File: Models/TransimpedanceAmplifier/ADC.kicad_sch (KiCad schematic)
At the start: 9 parts, among them U13 ADS8699

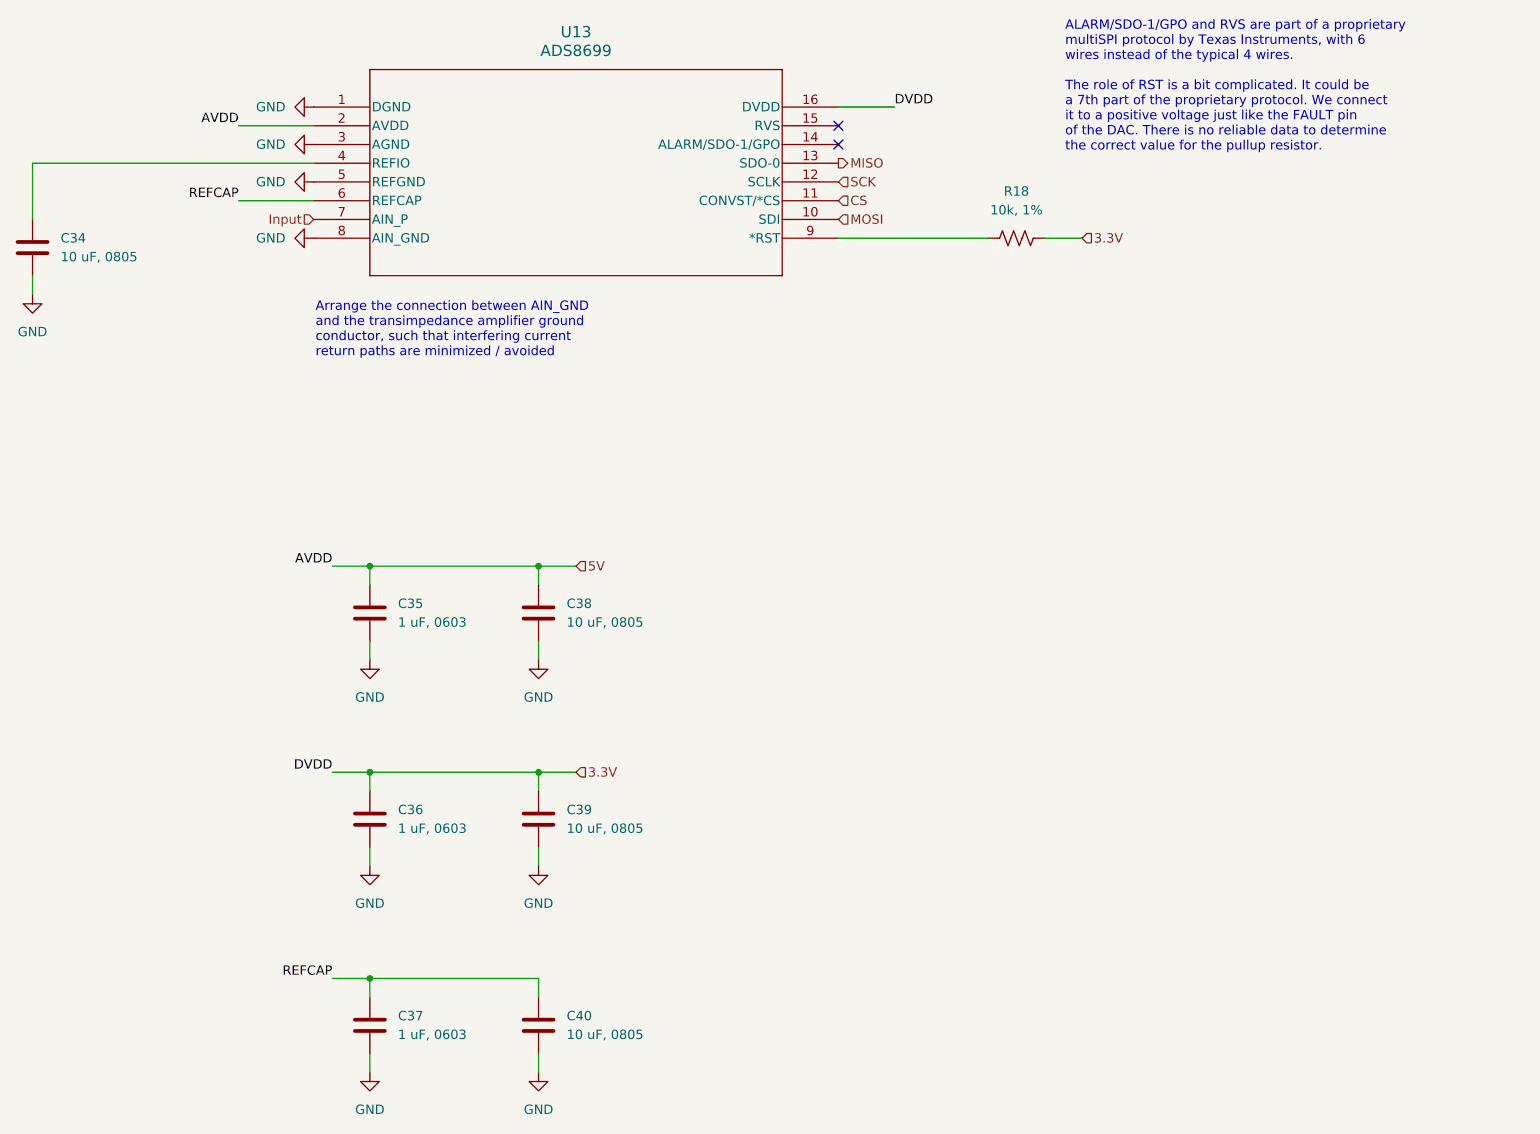
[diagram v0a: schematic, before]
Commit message: First successful ERC
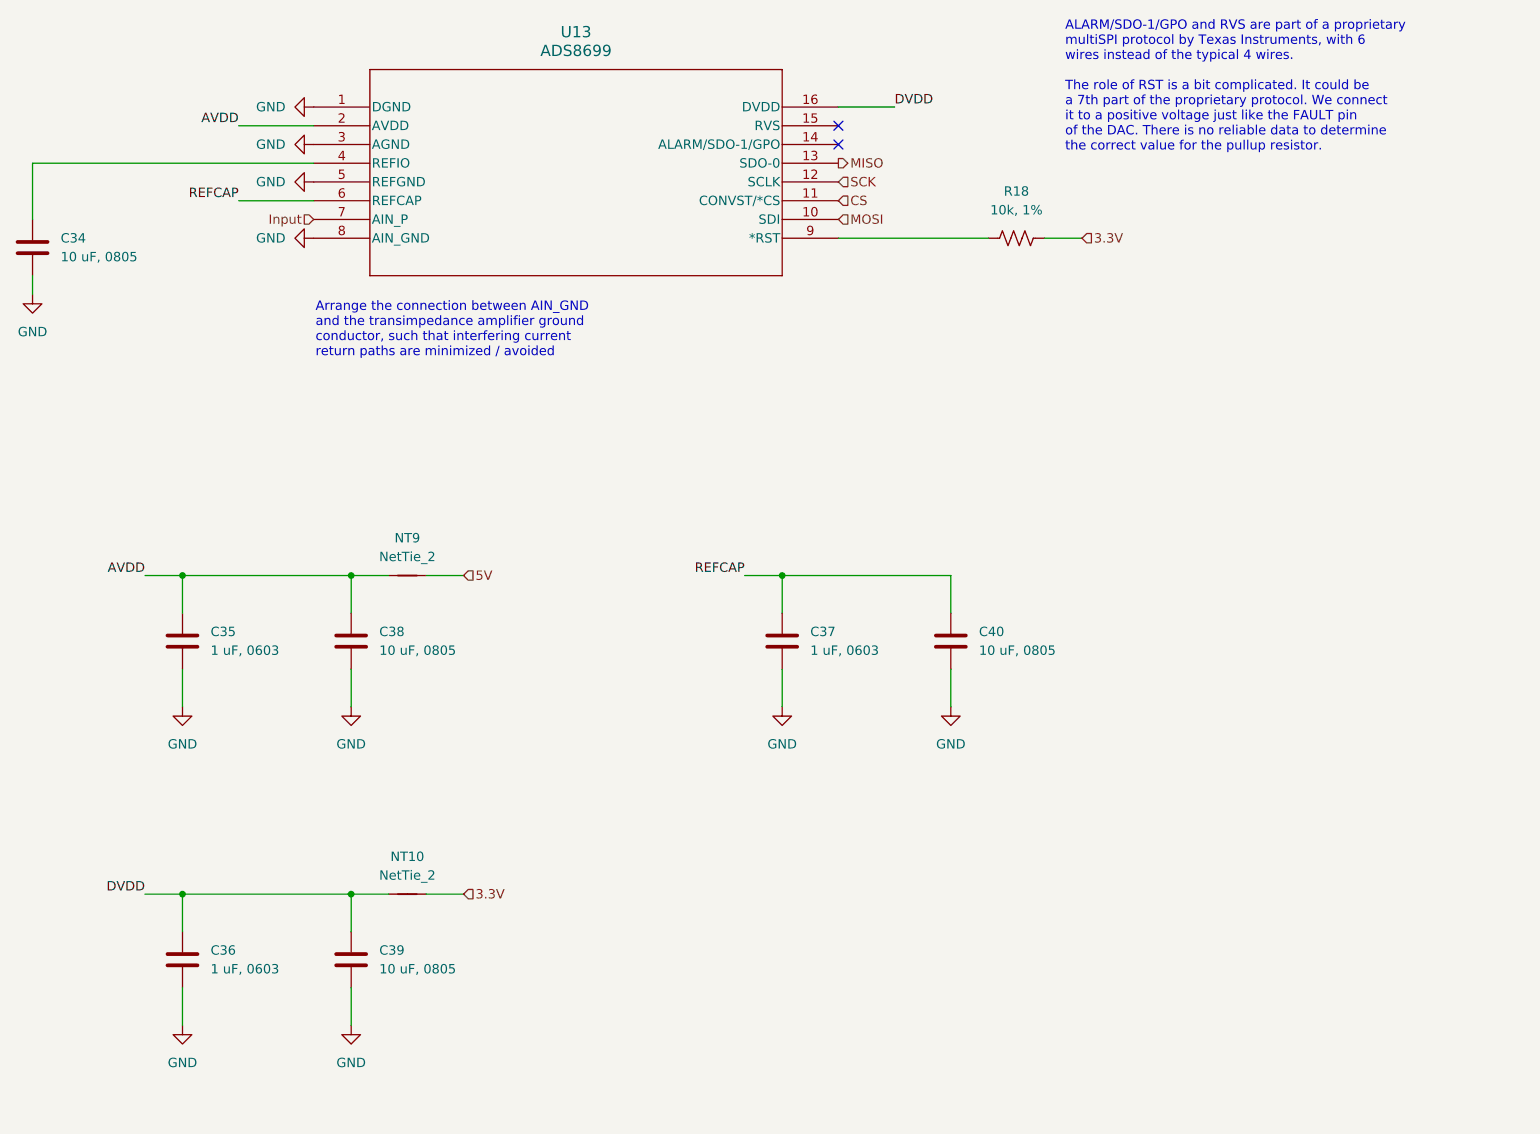
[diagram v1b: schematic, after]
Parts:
- added NT10, NT9: NetTie_2, symbol Device:NetTie_2
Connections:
- net 3.3V: now also NT10.2; no longer C36.1, C39.1, U13.16 (DVDD)
- net 5V: now also NT9.2; no longer C35.1, C38.1, U13.2 (AVDD)
- new net AVDD: C35.1, C38.1, NT9.1, U13.2 (AVDD)
- new net DVDD: C36.1, C39.1, NT10.1, U13.16 (DVDD)
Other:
- moved on the sheet: C35, C36, C37, C38, C39, C40
